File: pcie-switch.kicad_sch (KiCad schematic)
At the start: 1 part, among them U1 PI7C9X3G606GPCFCAEX

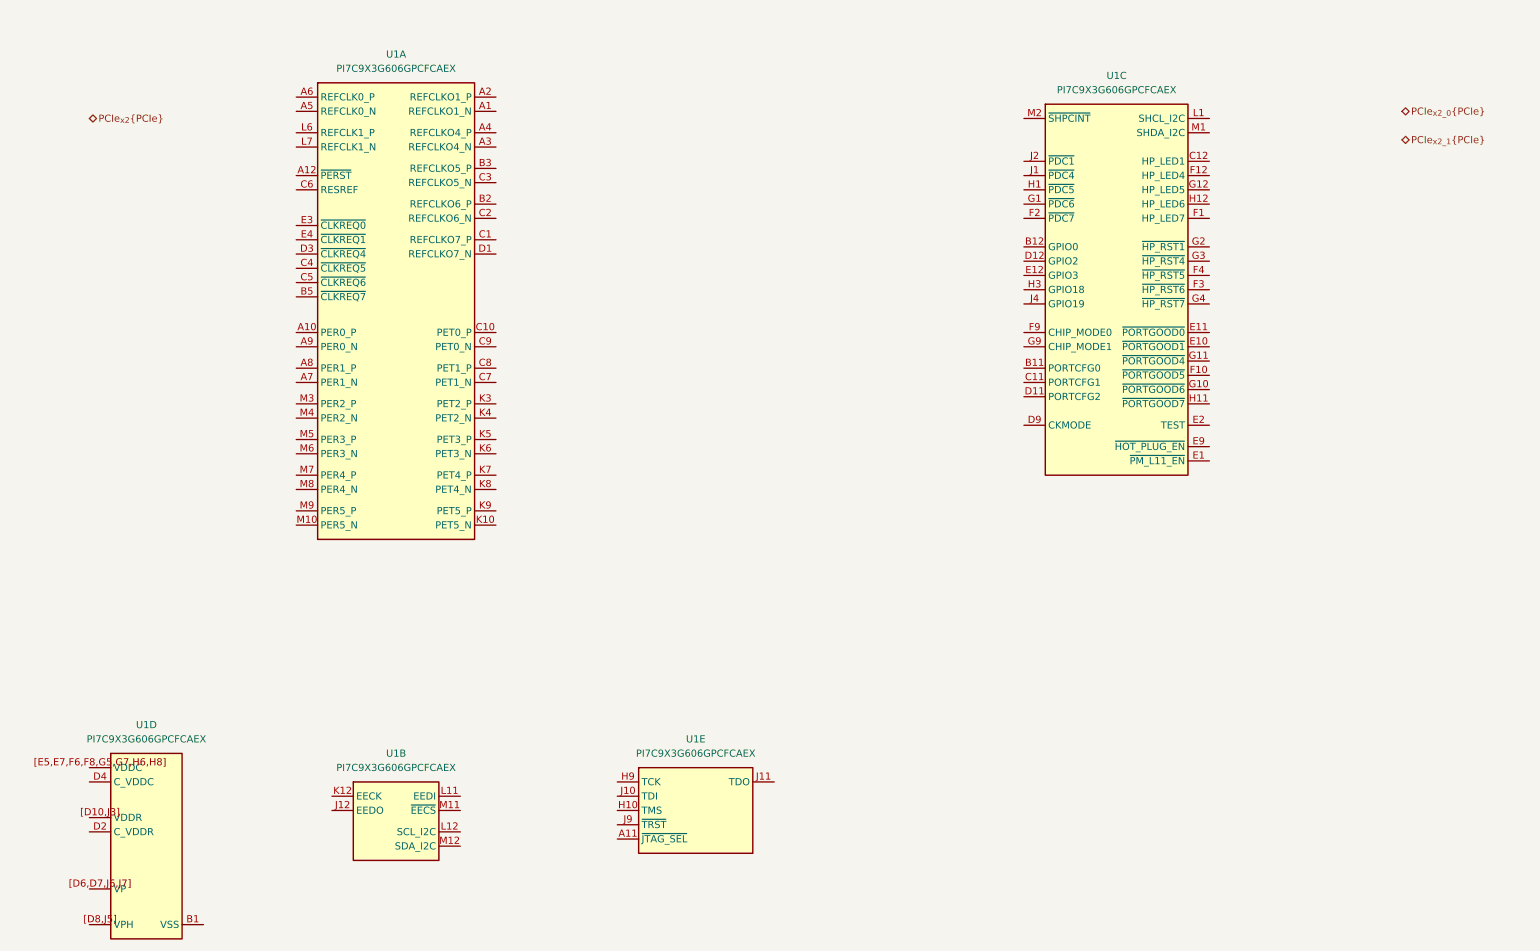
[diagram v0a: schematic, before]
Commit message: [#100765] Update symbol and tables
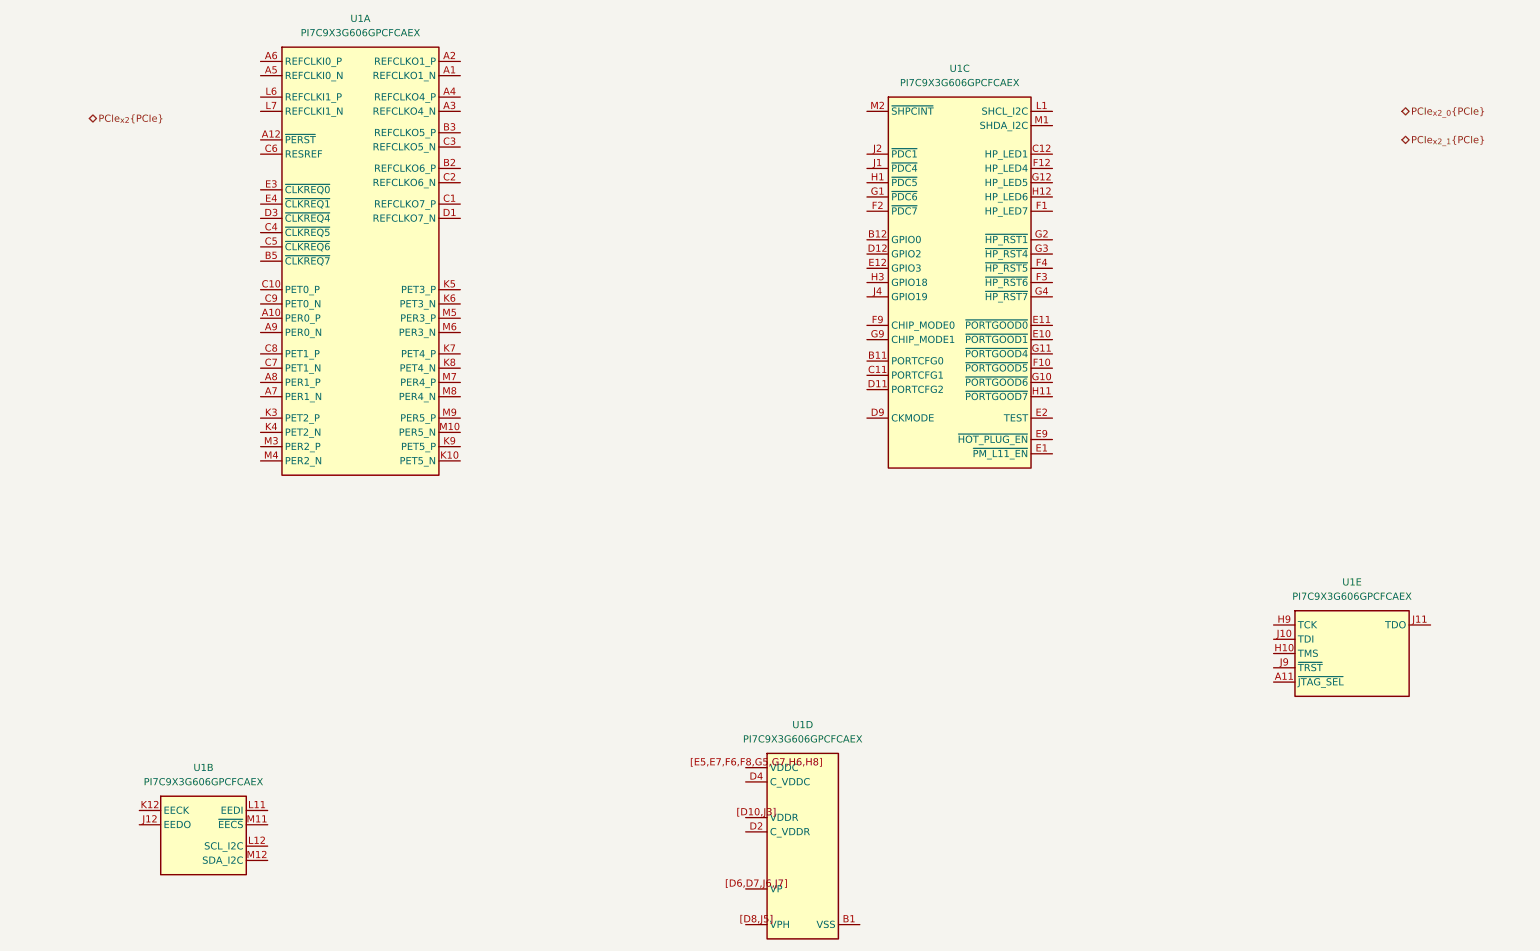
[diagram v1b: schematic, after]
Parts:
- removed U1: PI7C9X3G606GPCFCAEX, antmicro-footprints:BGA-144_10x10mm_Layout12x12_P0.8mm, symbol antmicroInterfaceControllers:PI7C9X3G606GPCFCAEX
- added U1: PI7C9X3G606GP, antmicro-footprints:BGA-144_10x10mm_Layout12x12_P0.8mm, symbol antmicroInterfaceControllers:PI7C9X3G606GP
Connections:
- new net: U1.B1 (VSS), U1.B10 (VSS), U1.B4 (VSS), U1.B6 (VSS), U1.B7 (VSS), U1.B8 (VSS), U1.B9 (VSS), U1.D5 (VSS), U1.E6 (VSS), U1.E8 (VSS), U1.F11 (VSS), U1.F5 (VSS), U1.F7 (VSS), U1.G6 (VSS), U1.G8 (VSS), U1.H5 (VSS), U1.H7 (VSS), U1.J8 (VSS), U1.K11 (VSS), U1.K2 (VSS), U1.L10 (VSS), U1.L3 (VSS), U1.L4 (VSS), U1.L5 (VSS), U1.L8 (VSS), U1.L9 (VSS)
